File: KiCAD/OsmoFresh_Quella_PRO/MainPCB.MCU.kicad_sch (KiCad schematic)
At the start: 22 parts, among them CN11 Conn_01x04_Pin, CN14 Conn_01x02_Pin, CN2 Conn_01x02_Pin, CN6 Conn_01x02_Pin, CN7 Conn_01x02_Pin, CN9 Conn_01x02_Pin

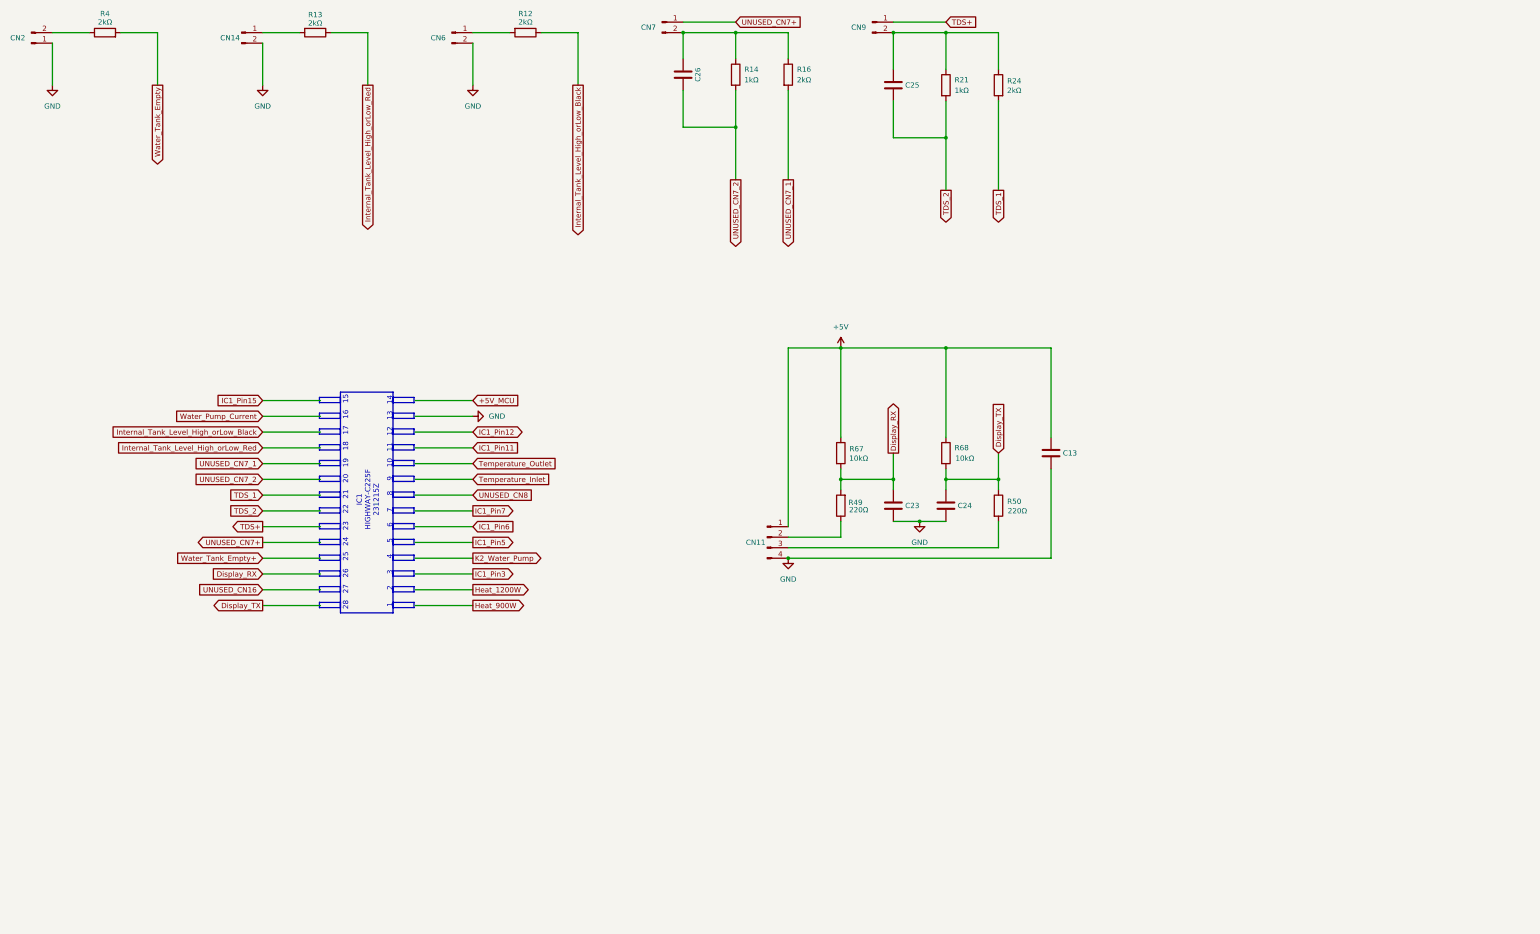
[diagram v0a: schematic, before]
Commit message: Update Schematics
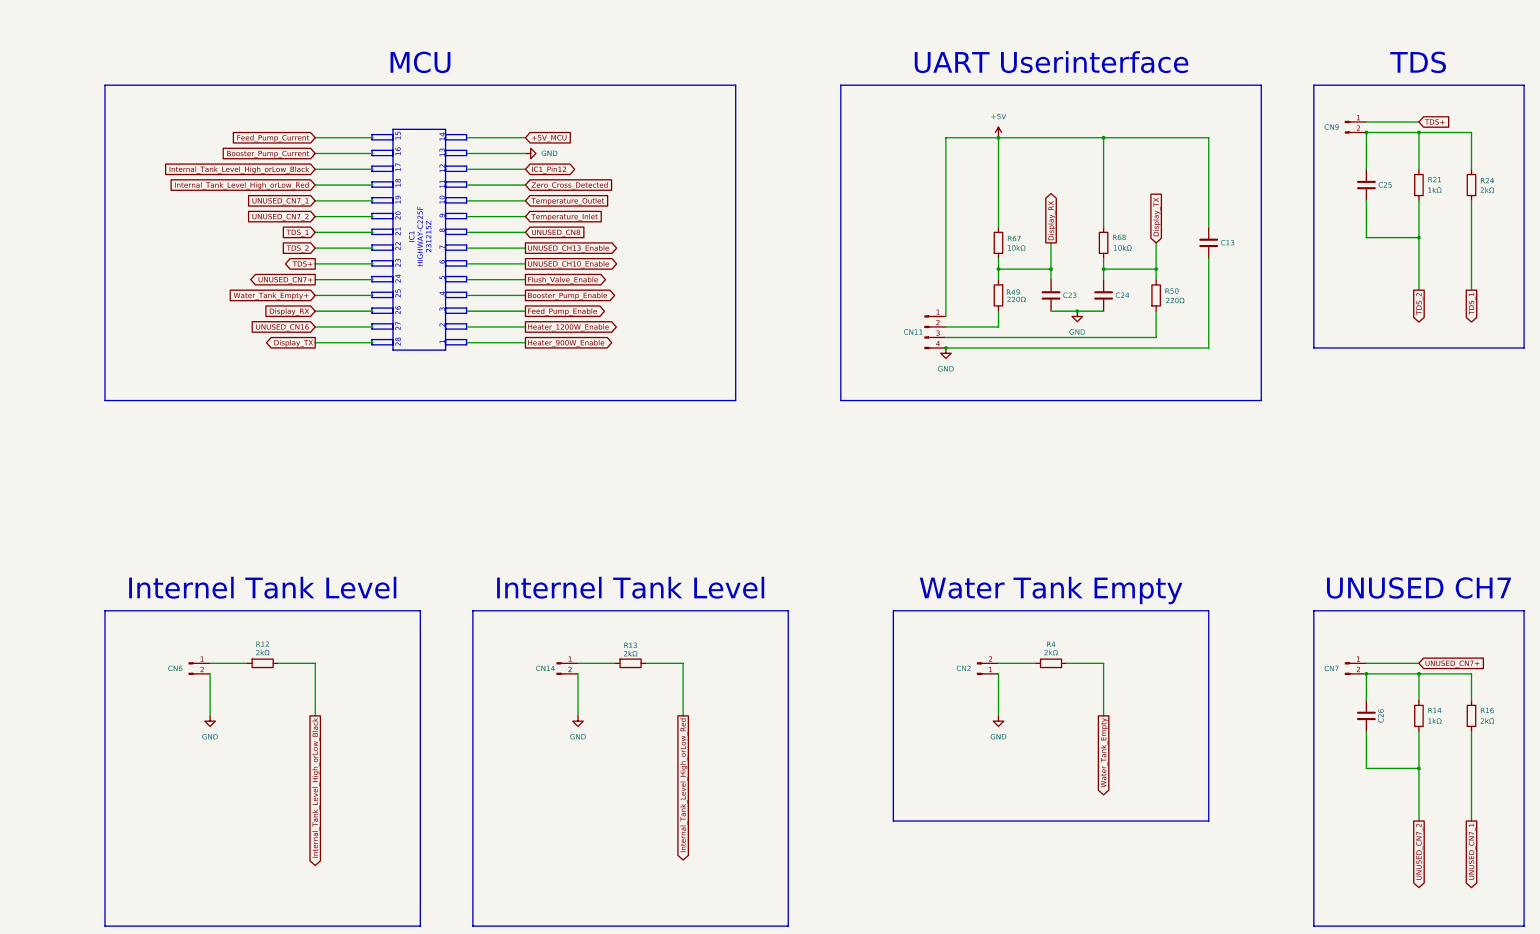
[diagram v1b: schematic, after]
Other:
- note added: "Internel Tank Level"
- note added: "MCU"
- note added: "TDS"
- note added: "UART Userinterface"
- note added: "UNUSED CH7"
- note added: "Water Tank Empty"
- moved on the sheet: C13, C23, C24, C25, C26, CN11, CN14, CN2, CN6, CN7, CN9, R12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
